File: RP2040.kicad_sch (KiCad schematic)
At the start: 39 parts, among them J1 USB_C_Receptacle_USB2.0_14P, J2 Conn_01x20, J3 Conn_01x20, J4 Conn_01x03, SW1 SW_Push, U1 RP2040, U2 MCP1700x-330xxTT, U4 W25Q16JVUXIQ TR, Y1 12 MHz

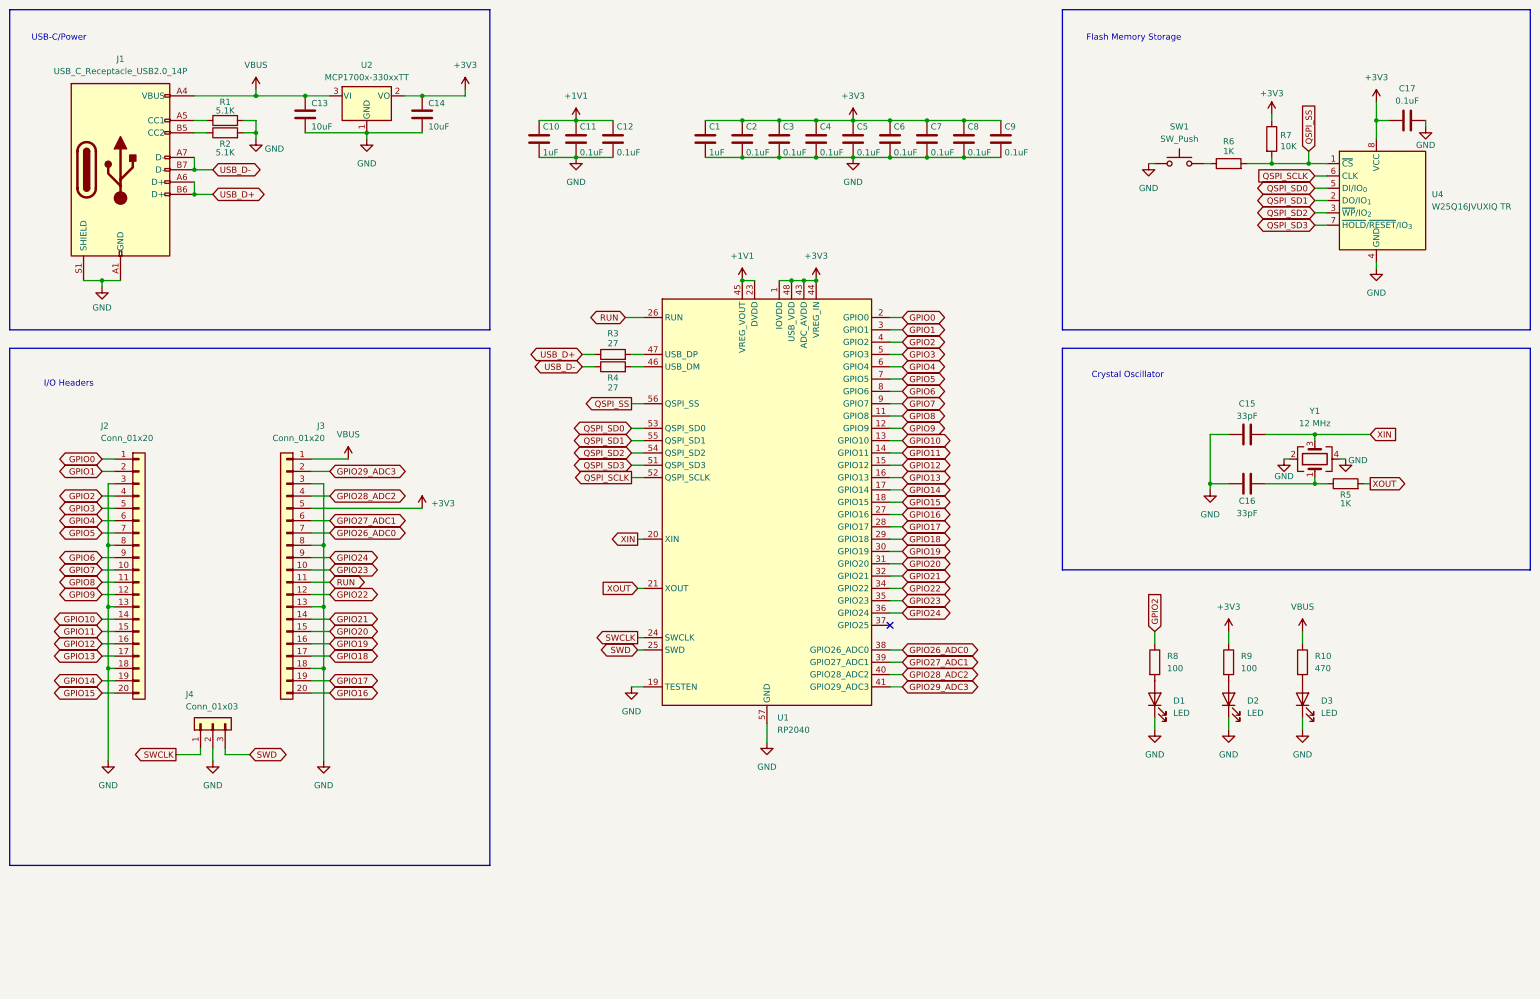
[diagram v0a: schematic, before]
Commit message: Update Readme + Images
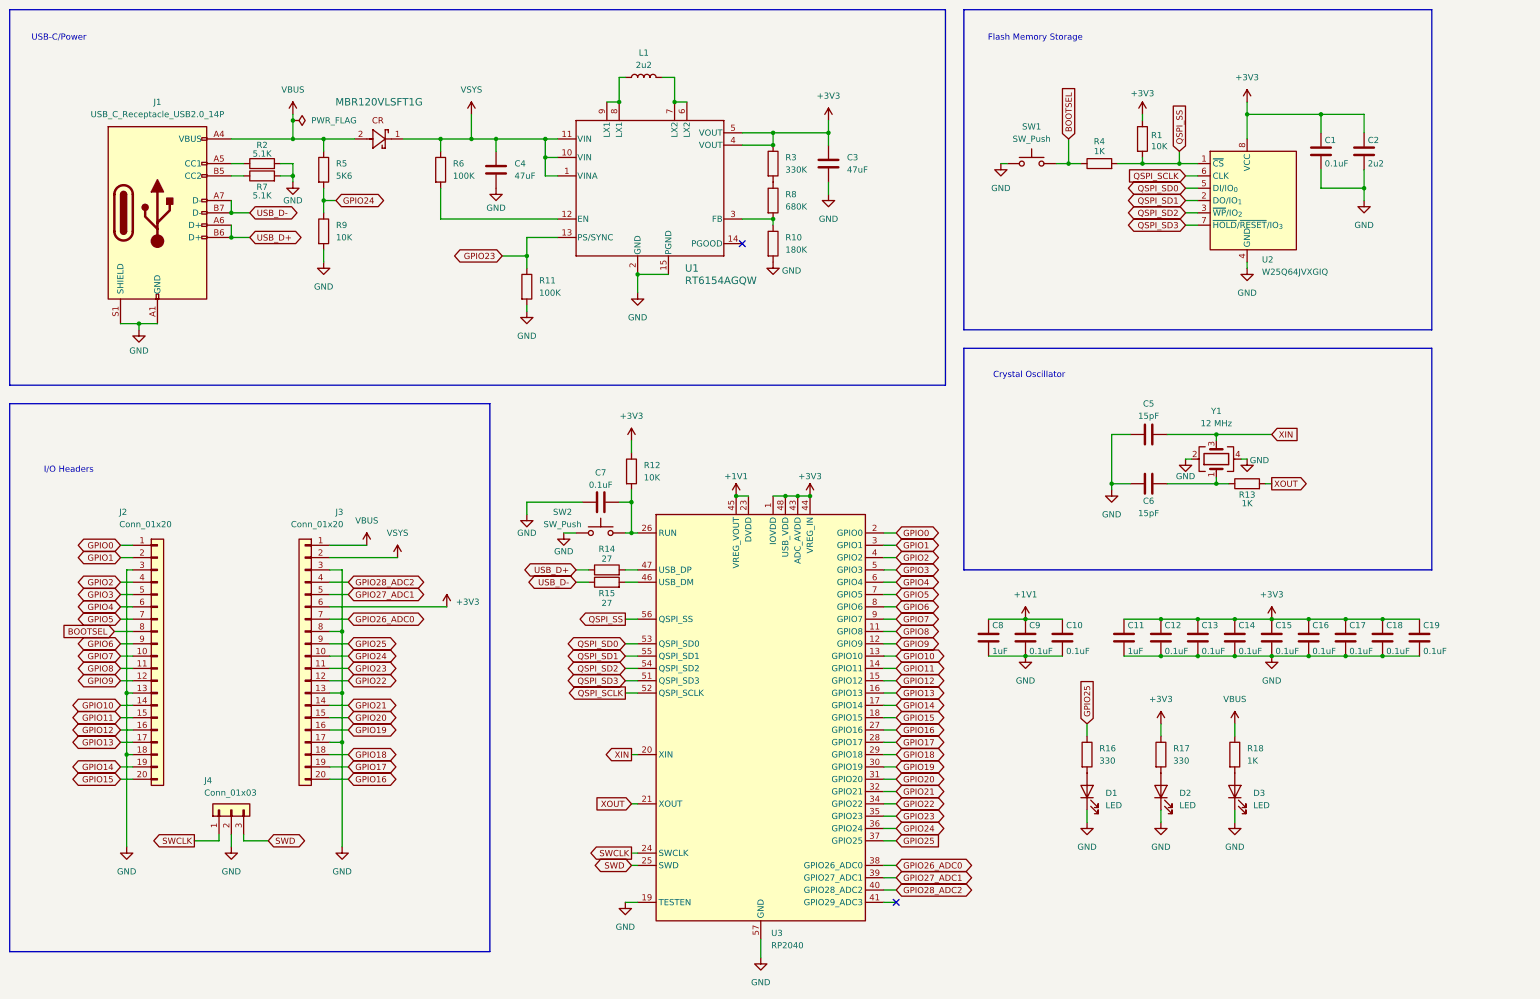
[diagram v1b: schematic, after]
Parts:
- removed C13, C14: 10uF, Capacitor_SMD:C_0603_1608Metric, symbol Device:C
- removed C17: 0.1uF, Capacitor_SMD:C_0402_1005Metric, symbol Device:C
- removed R1: 5.1K, Resistor_SMD:R_0402_1005Metric, symbol Device:R
- removed U2: MCP1700x-330xxTT, Package_TO_SOT_SMD:SOT-23, symbol Regulator_Linear:MCP1700x-330xxTT
- added 111111111: MBR120VLSFT1G, RP2040:SDO_SOD-123FL_ONS, symbol Schottky_Diodes:MBR120VLSFT1G
- added C1, C7: 0.1uF, Capacitor_SMD:C_0402_1005Metric, symbol Device:C
- added C2: 2u2, Capacitor_SMD:C_0603_1608Metric, symbol Device:C
- added C3, C4: 47uF, Capacitor_SMD:C_0805_2012Metric, symbol Device:C
- added L1: 2u2, Inductor_SMD:L_1008_2520Metric, symbol Device:L
- added R10: 180K, Resistor_SMD:R_0402_1005Metric, symbol Device:R
- added R11, R6: 100K, Resistor_SMD:R_0402_1005Metric, symbol Device:R
- added R12, R9: 10K, Resistor_SMD:R_0402_1005Metric, symbol Device:R
- added R2: 5.1K, Resistor_SMD:R_0402_1005Metric, symbol Device:R
- added R3: 330K, Resistor_SMD:R_0402_1005Metric, symbol Device:R
- added R5: 5K6, Resistor_SMD:R_0402_1005Metric, symbol Device:R
- added R8: 680K, Resistor_SMD:R_0402_1005Metric, symbol Device:R
- added SW2: SW_Push, Button_Switch_SMD:SW_Push_SPST_NO_Alps_SKRK, symbol Switch:SW_Push
- added U1: RT6154AGQW, easyeda2kicad:VSON-14_L4.0-W3.0-P0.50-BL-EP_TI_DSJ, symbol RT6154A:RT6154AGQW
- C5: renamed from C15; value 33pF -> 15pF
- C6: renamed from C16; value 33pF -> 15pF
- R16: renamed from R8; value 100 -> 330
- R17: renamed from R9; value 100 -> 330
- R18: renamed from R10; value 470 -> 1K
- U2: renamed from U4; value W25Q16JVUXIQ TR -> W25Q64JVXGIQ; footprint Package_SON:Winbond_USON-8-1EP_3x2mm_P0.5mm_EP0.2x1.6mm -> easyeda2kicad:XSON-8_L4.0-W4.0-P0.80-TL-EP
- renumbered C12 to C10, C1 to C11, C2 to C12, C3 to C13, C4 to C14, C5 to C15, C6 to C16, C7 to C17, C8 to C18, C9 to C19, C10 to C8, C11 to C9, R7 to R1, R5 to R13, R3 to R14, R4 to R15, R6 to R4, R2 to R7, U1 to U3
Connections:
- net +3V3: now also J3.6 (Pin_6), C1.1, C2.1, C3.1, R12.1, R3.1, U1.4 (VOUT), U1.5 (VOUT); no longer J3.5 (Pin_5)
- net GND: now also J3.17 (Pin_17), C1.2, C2.2, C3.2, C4.2, C7.1, R10.2, R11.2, R2.2, R9.2, SW2.1, U1.15 (PGND), U1.2 (GND); no longer J2.8 (Pin_8), J3.18 (Pin_18)
- net GPIO18: now also J3.18 (Pin_18); no longer J3.17 (Pin_17)
- net GPIO2: no longer R16.1
- net GPIO23: now also J3.11 (Pin_11), R11.1, U1.13 (PS/SYNC); no longer J3.10 (Pin_10)
- net GPIO24: now also J3.10 (Pin_10), R5.2, R9.1; no longer J3.9 (Pin_9)
- net GPIO27_ADC1: now also J3.5 (Pin_5); no longer J3.6 (Pin_6)
- net VBUS: now also 111111111.2, R5.1
- net GPIO25: now reaches U3.37 (GPIO25)
- net GPIO25: now also J3.9 (Pin_9), R16.1
- net at J1.A5 (CC1): now also R2.1
- net BOOTSEL: now reaches R4.1, SW1.2
- net BOOTSEL: now also J2.8 (Pin_8)
- net GPIO29_ADC3: no longer names the net of U3.41 (GPIO29_ADC3)
- net GPIO29_ADC3: no longer J3.2 (Pin_2)
- net RUN: no longer names the net of U3.26 (RUN)
- net RUN: now also C7.2, R12.2, SW2.2; no longer J3.11 (Pin_11)
- new net: R6.2, U1.12 (EN)
- new net: L1.1, U1.8 (LX1), U1.9 (LX1)
- new net: L1.2, U1.6 (LX2), U1.7 (LX2)
- new net: R10.1, R8.2, U1.3 (FB)
- new net: R3.2, R8.1
- new net VSYS: 111111111.1, C4.1, J3.2 (Pin_2), R6.1, U1.1 (VINA), U1.10 (VIN), U1.11 (VIN)
- no-connect marks 1 -> 2
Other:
- moved on the sheet: C10, C11, C12, C13, C14, C15, C16, C17, C18, C19, C5, C6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
